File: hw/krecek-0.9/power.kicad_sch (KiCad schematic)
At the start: 58 parts, among them J3 USB_C_Receptacle_USB2.0, Q1 AO3401A, Q2 AO3401A, Q3 AO3400A, Q4 AO3400A, Q5 AO3400A, Q6 AO3400A, U10 TPS63000, U5 AMS1117-3.3, U6 JST-PH-2P, U7 BQ24040DSQR, U8 AMS1117-3.3, U9 AMS1117-3.3

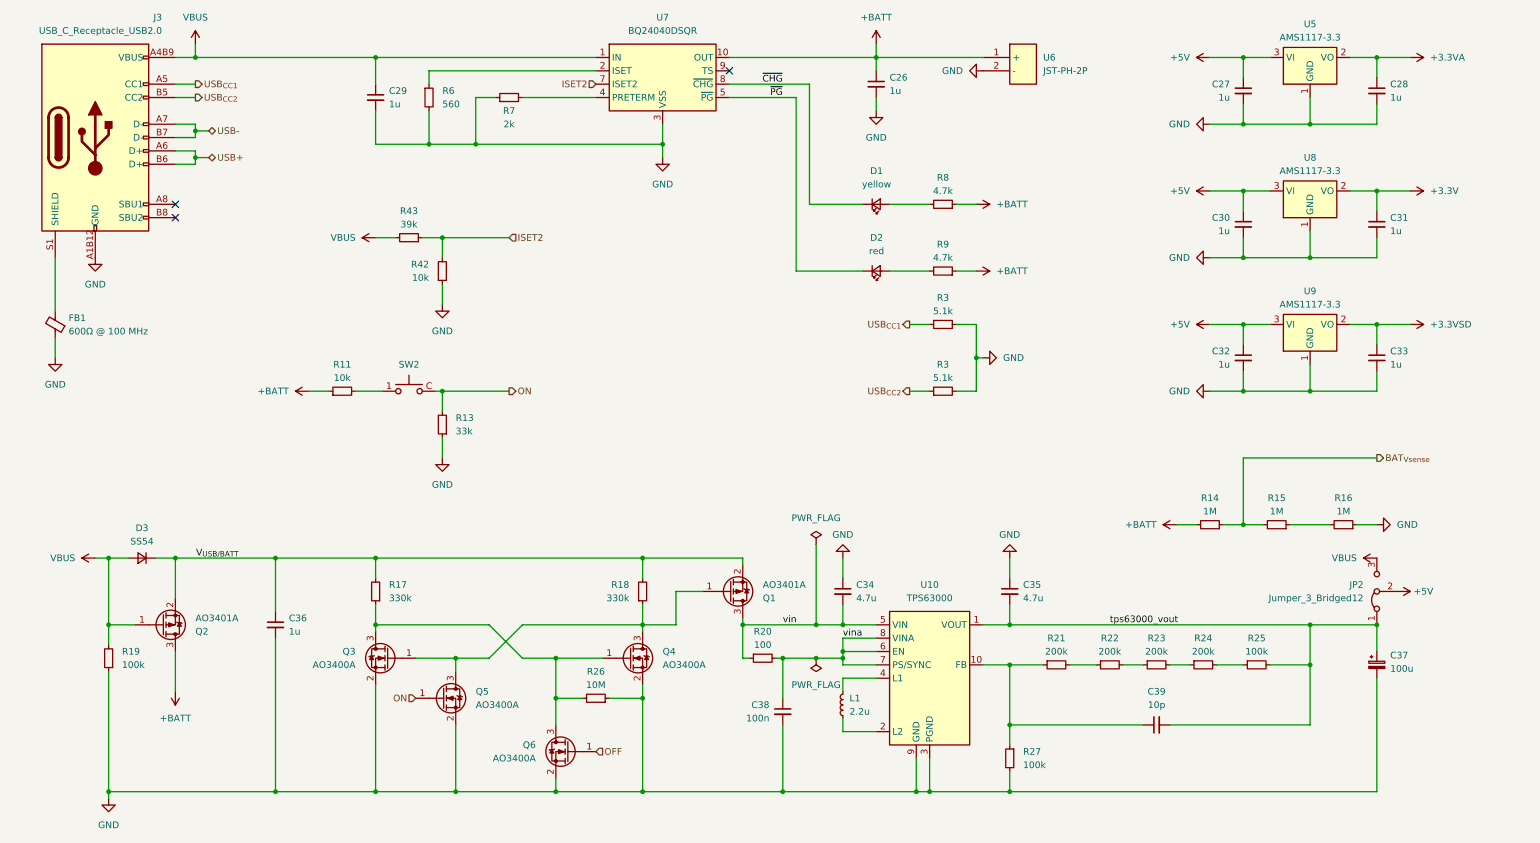
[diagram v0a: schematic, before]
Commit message: Improve flip-flop design
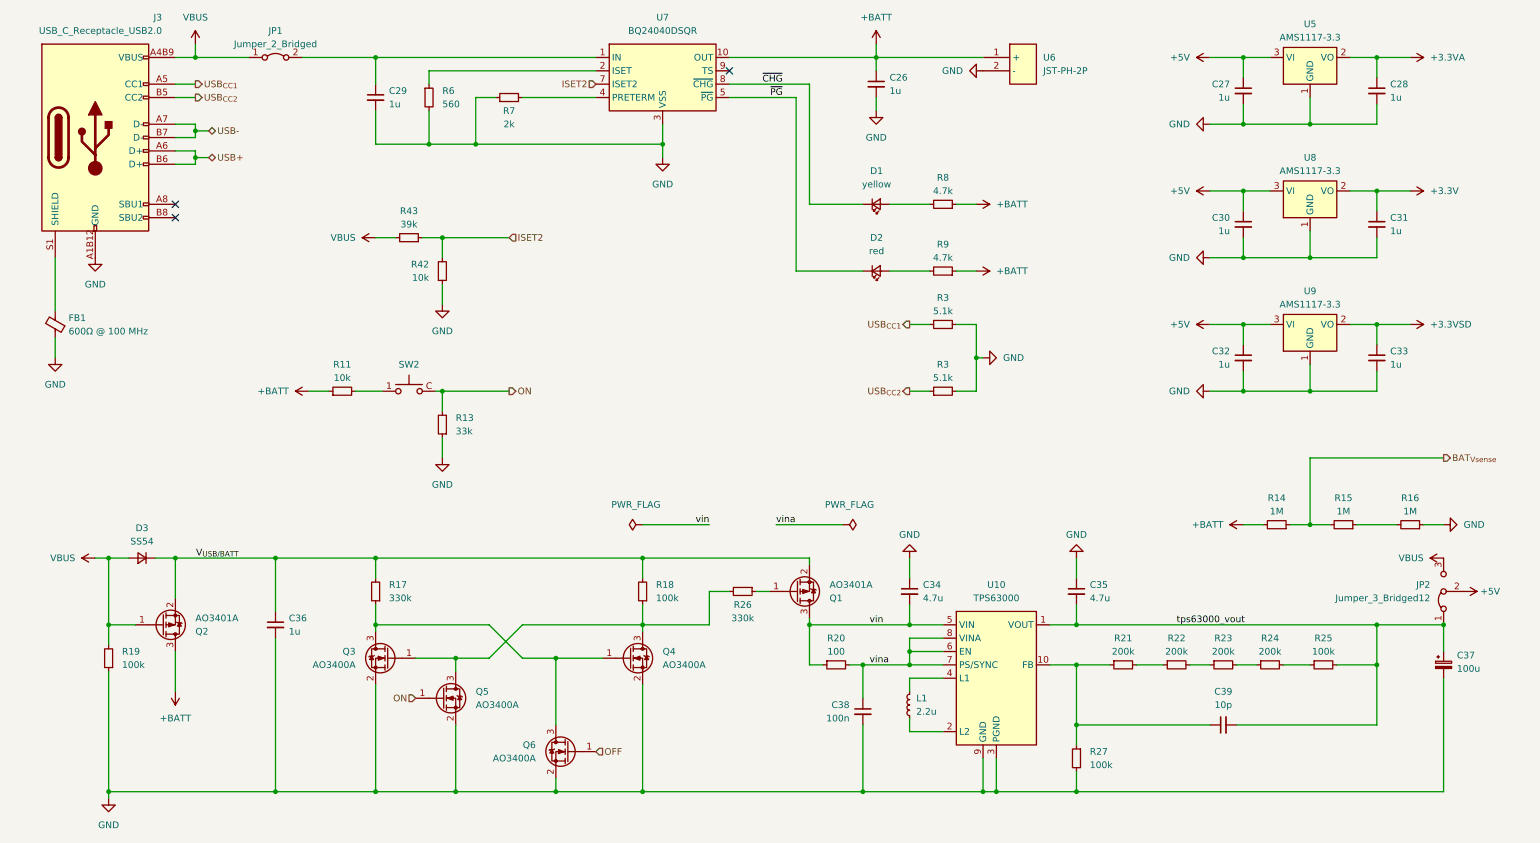
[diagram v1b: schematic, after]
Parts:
- added JP1: Jumper_2_Bridged, Jumper:SolderJumper-2_P1.3mm_Bridged_RoundedPad1.0x1.5mm, symbol Jumper:Jumper_2_Bridged
- R18: value 330k -> 100k; footprint Resistor_SMD:R_0603_1608Metric -> Resistor_SMD:R_0402_1005Metric; LCSC Part C23137 -> C25741
- R26: value 10M -> 330k; LCSC Part C7250 -> C23137
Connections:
- net GND: no longer R26.1
- net VBUS: now also JP1.1 (A); no longer C29.1, U7.1 (IN)
- net at Q3.1 (G), Q4.3 (D), Q5.3 (D)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: now also R26.2; no longer Q1.1 (G)
- net at Q3.3 (D), Q4.1 (G), Q6.3 (D)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: no longer R26.2
- new net: C29.1, JP1.2 (B), U7.1 (IN)
- new net: Q1.1 (G), R26.1
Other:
- moved on the sheet: C34, C35, C37, C38, C39, JP2, L1, Q1, R14, R15, R16, R20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
